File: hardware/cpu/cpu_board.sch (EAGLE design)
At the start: 53 parts, among them IC4 7404N, IC5 7400N, IC6 74HCT139N, IC7 7400N, IC9 74HCT138N, X1 22-23-2041

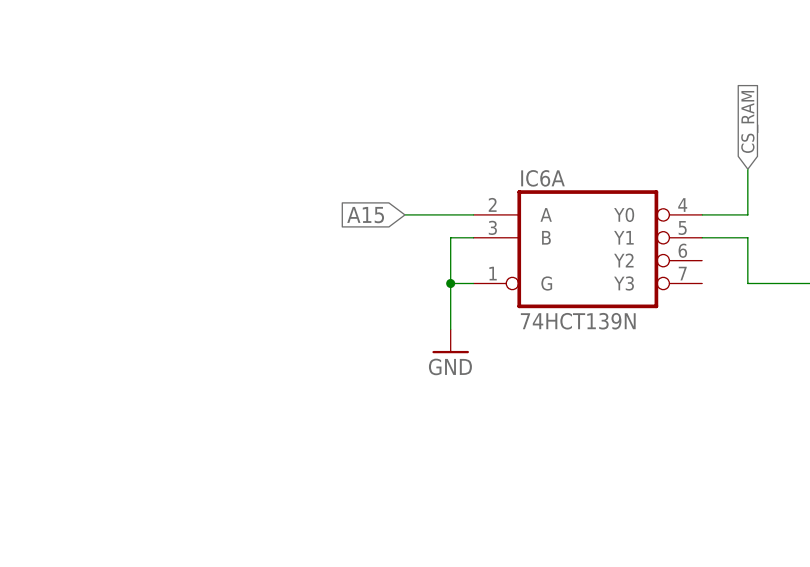
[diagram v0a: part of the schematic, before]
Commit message: AEN signal connected to memory address decoder
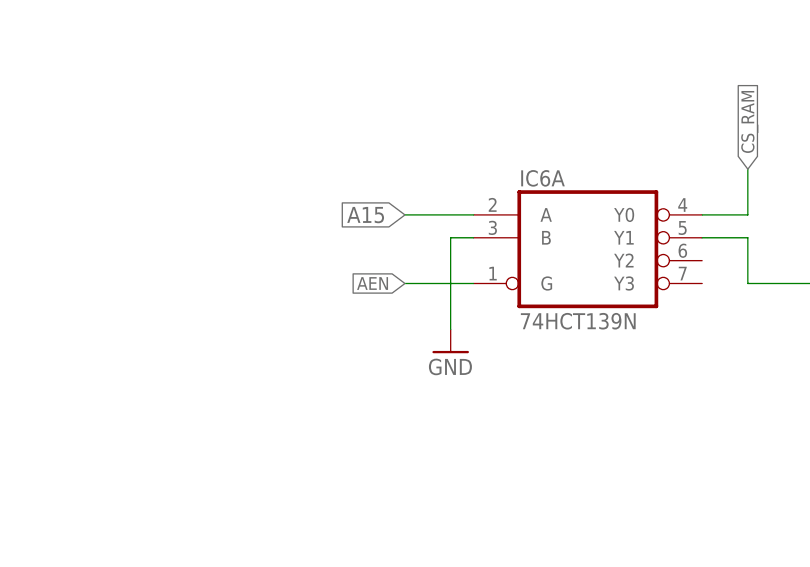
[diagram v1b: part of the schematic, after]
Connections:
- net AEN: now also IC6A.G
- net GND: no longer IC6A.G
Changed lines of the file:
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@@
 <pinref part="GND10" gate="1" pin="GND"/>
 <wire x1="10.16" y1="-147.32" x2="7.62" y2="-147.32" width="0.1524" layer="91"/>
-<wire x1="7.62" y1="-147.32" x2="7.62" y2="-152.4" width="0.1524" layer="91"/>
-<pinref part="IC6" gate="A" pin="G"/>
-<wire x1="7.62" y1="-152.4" x2="7.62" y2="-157.48" width="0.1524" layer="91"/>
-<wire x1="10.16" y1="-152.4" x2="7.62" y2="-152.4" width="0.1524" layer="91"/>
-<junction x="7.62" y="-152.4"/>
+<wire x1="7.62" y1="-147.32" x2="7.62" y2="-157.48" width="0.1524" layer="91"/>
 </segment>
 <segment>
@@
 <wire x1="116.84" y1="-147.32" x2="114.3" y2="-147.32" width="0.1524" layer="91"/>
 </segment>
-</net>
+<segment>
+<pinref part="IC6" gate="A" pin="G"/>
+<wire x1="10.16" y1="-152.4" x2="2.54" y2="-152.4" width="0.1524" layer="91"/>
+<label x="2.54" y="-152.4" size="1.4224" layer="95" rot="R180" xref="yes"/>
+</segment>
+</net>

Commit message: AEN removed from memory address decoder
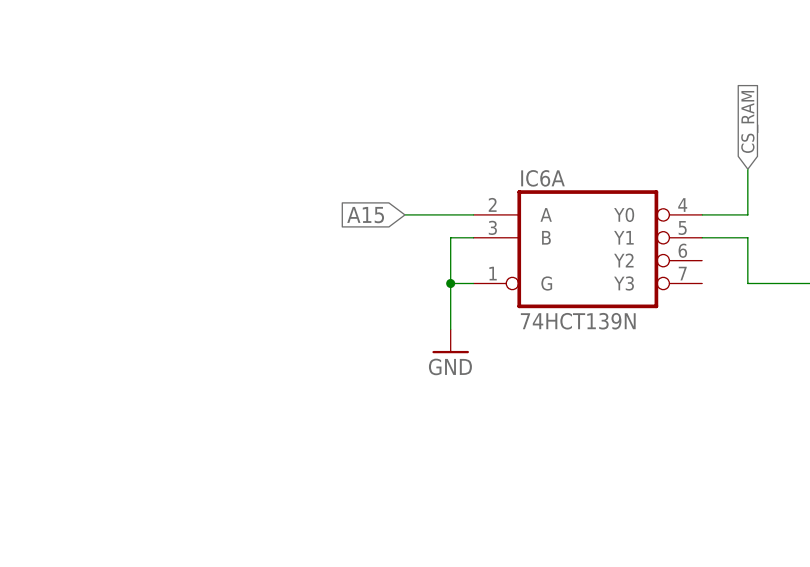
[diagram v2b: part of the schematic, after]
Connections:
- net AEN: no longer IC6A.G
- net GND: now also IC6A.G
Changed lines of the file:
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@@
 <pinref part="GND10" gate="1" pin="GND"/>
 <wire x1="10.16" y1="-147.32" x2="7.62" y2="-147.32" width="0.1524" layer="91"/>
-<wire x1="7.62" y1="-147.32" x2="7.62" y2="-157.48" width="0.1524" layer="91"/>
+<wire x1="7.62" y1="-147.32" x2="7.62" y2="-152.4" width="0.1524" layer="91"/>
+<pinref part="IC6" gate="A" pin="G"/>
+<wire x1="7.62" y1="-152.4" x2="7.62" y2="-157.48" width="0.1524" layer="91"/>
+<wire x1="10.16" y1="-152.4" x2="7.62" y2="-152.4" width="0.1524" layer="91"/>
+<junction x="7.62" y="-152.4"/>
 </segment>
 <segment>
@@
 <wire x1="116.84" y1="-147.32" x2="114.3" y2="-147.32" width="0.1524" layer="91"/>
 </segment>
-<segment>
-<pinref part="IC6" gate="A" pin="G"/>
-<wire x1="10.16" y1="-152.4" x2="2.54" y2="-152.4" width="0.1524" layer="91"/>
-<label x="2.54" y="-152.4" size="1.4224" layer="95" rot="R180" xref="yes"/>
-</segment>
-</net>
+</net>
